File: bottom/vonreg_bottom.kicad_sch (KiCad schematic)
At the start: 8 parts, among them J1 AudioJack4, T1 SW_Push, T2 SW_Push, T3 SW_Push

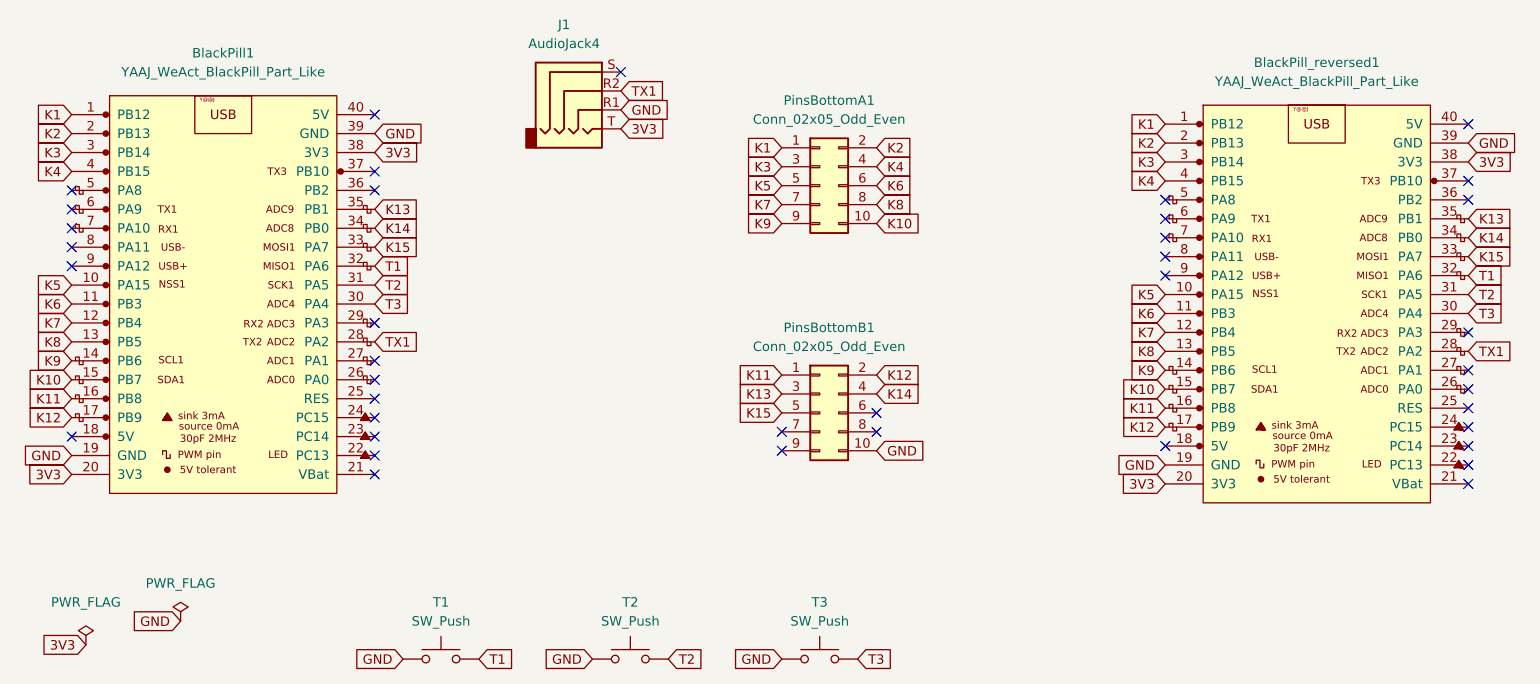
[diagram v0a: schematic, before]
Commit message: Routing done, hopefully
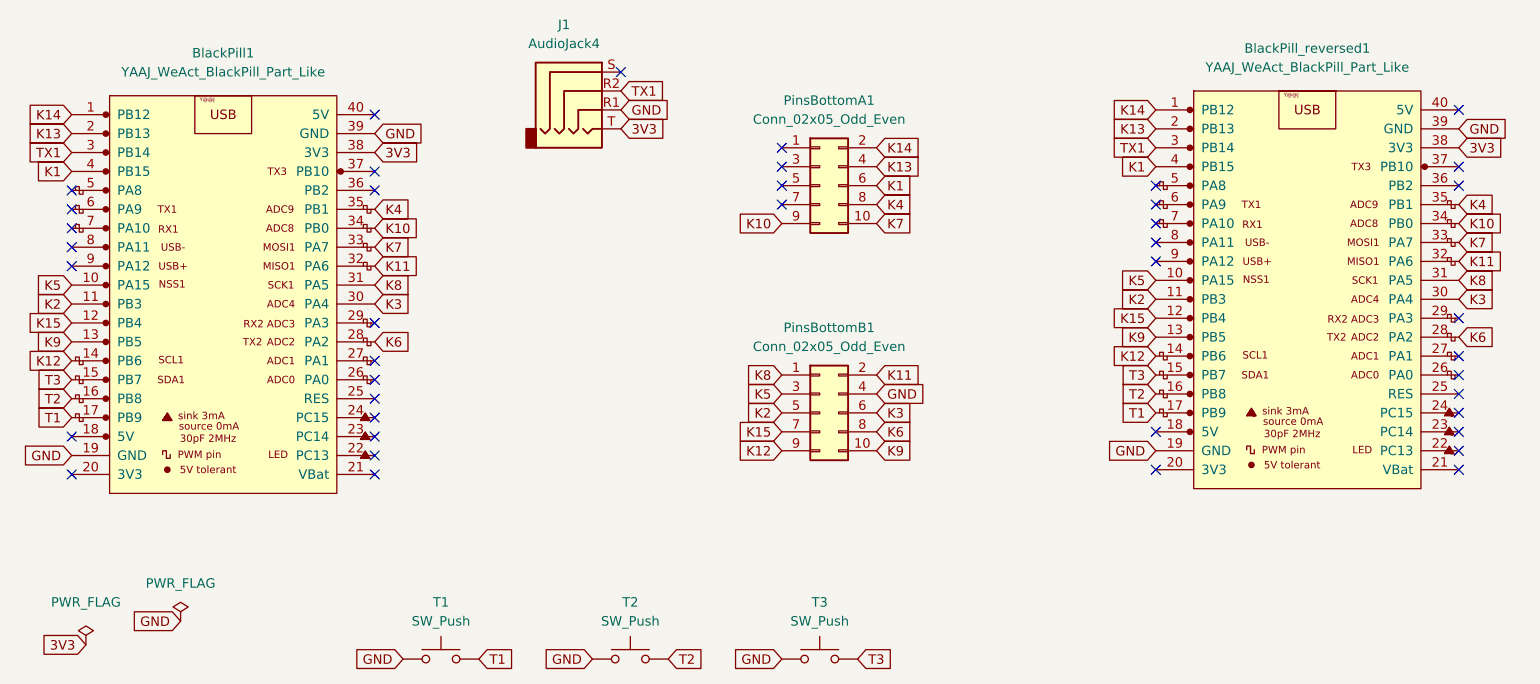
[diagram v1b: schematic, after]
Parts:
- J1: footprint keebio:TRRS-PJ-320A-dual -> Connector_Audio:TRRS-PJ-320A-dual
- T1, T2, T3: footprint Button_Switch_Keyboard:SW_Cherry_MX_1.00u_PCB -> Button_Switch_Keyboard:Kailh_socket_MX_optional_reversible
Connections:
- net 3V3: no longer BlackPill1.20 (3V3), BlackPill_reversed1.20 (3V3)
- net GND: now also PinsBottomB1.4 (Pin_4); no longer PinsBottomB1.10 (Pin_10)
- net K1: now also BlackPill1.4 (PB15), BlackPill_reversed1.4 (PB15), PinsBottomA1.6 (Pin_6); no longer BlackPill1.1 (PB12), BlackPill_reversed1.1 (PB12), PinsBottomA1.1 (Pin_1)
- net K10: now also BlackPill1.34 (PB0), BlackPill_reversed1.34 (PB0), PinsBottomA1.9 (Pin_9); no longer BlackPill1.15 (PB7), BlackPill_reversed1.15 (PB7), PinsBottomA1.10 (Pin_10)
- net K11: now also BlackPill1.32 (PA6), BlackPill_reversed1.32 (PA6), PinsBottomB1.2 (Pin_2); no longer BlackPill1.16 (PB8), BlackPill_reversed1.16 (PB8), PinsBottomB1.1 (Pin_1)
- net K12: now also BlackPill1.14 (PB6), BlackPill_reversed1.14 (PB6), PinsBottomB1.9 (Pin_9); no longer BlackPill1.17 (PB9), BlackPill_reversed1.17 (PB9), PinsBottomB1.2 (Pin_2)
- net K13: now also BlackPill1.2 (PB13), BlackPill_reversed1.2 (PB13), PinsBottomA1.4 (Pin_4); no longer BlackPill1.35 (PB1), BlackPill_reversed1.35 (PB1), PinsBottomB1.3 (Pin_3)
- net K14: now also BlackPill1.1 (PB12), BlackPill_reversed1.1 (PB12), PinsBottomA1.2 (Pin_2); no longer BlackPill1.34 (PB0), BlackPill_reversed1.34 (PB0), PinsBottomB1.4 (Pin_4)
- net K15: now also BlackPill1.12 (PB4), BlackPill_reversed1.12 (PB4), PinsBottomB1.7 (Pin_7); no longer BlackPill1.33 (PA7), BlackPill_reversed1.33 (PA7), PinsBottomB1.5 (Pin_5)
- net K2: now also BlackPill1.11 (PB3), BlackPill_reversed1.11 (PB3), PinsBottomB1.5 (Pin_5); no longer BlackPill1.2 (PB13), BlackPill_reversed1.2 (PB13), PinsBottomA1.2 (Pin_2)
- net K3: now also BlackPill1.30 (PA4), BlackPill_reversed1.30 (PA4), PinsBottomB1.6 (Pin_6); no longer BlackPill1.3 (PB14), BlackPill_reversed1.3 (PB14), PinsBottomA1.3 (Pin_3)
- net K4: now also BlackPill1.35 (PB1), BlackPill_reversed1.35 (PB1), PinsBottomA1.8 (Pin_8); no longer BlackPill1.4 (PB15), BlackPill_reversed1.4 (PB15), PinsBottomA1.4 (Pin_4)
- net K5: now also PinsBottomB1.3 (Pin_3); no longer PinsBottomA1.5 (Pin_5)
- net K6: now also BlackPill1.28 (PA2), BlackPill_reversed1.28 (PA2), PinsBottomB1.8 (Pin_8); no longer BlackPill1.11 (PB3), BlackPill_reversed1.11 (PB3), PinsBottomA1.6 (Pin_6)
- net K7: now also BlackPill1.33 (PA7), BlackPill_reversed1.33 (PA7), PinsBottomA1.10 (Pin_10); no longer BlackPill1.12 (PB4), BlackPill_reversed1.12 (PB4), PinsBottomA1.7 (Pin_7)
- net K8: now also BlackPill1.31 (PA5), BlackPill_reversed1.31 (PA5), PinsBottomB1.1 (Pin_1); no longer BlackPill1.13 (PB5), BlackPill_reversed1.13 (PB5), PinsBottomA1.8 (Pin_8)
- net K9: now also BlackPill1.13 (PB5), BlackPill_reversed1.13 (PB5), PinsBottomB1.10 (Pin_10); no longer BlackPill1.14 (PB6), BlackPill_reversed1.14 (PB6), PinsBottomA1.9 (Pin_9)
- net T1: now also BlackPill1.17 (PB9), BlackPill_reversed1.17 (PB9); no longer BlackPill1.32 (PA6), BlackPill_reversed1.32 (PA6)
- net T2: now also BlackPill1.16 (PB8), BlackPill_reversed1.16 (PB8); no longer BlackPill1.31 (PA5), BlackPill_reversed1.31 (PA5)
- net T3: now also BlackPill1.15 (PB7), BlackPill_reversed1.15 (PB7); no longer BlackPill1.30 (PA4), BlackPill_reversed1.30 (PA4)
- net TX1: now also BlackPill1.3 (PB14), BlackPill_reversed1.3 (PB14); no longer BlackPill1.28 (PA2), BlackPill_reversed1.28 (PA2)
- no-connect marks 39 -> 41
